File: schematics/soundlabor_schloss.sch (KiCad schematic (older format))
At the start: 18 parts, among them P1 CONN_01X03, P2 CONN_01X02, P3 CONN_01X02, Q1 Q_NMOS_GDS, U1 4538

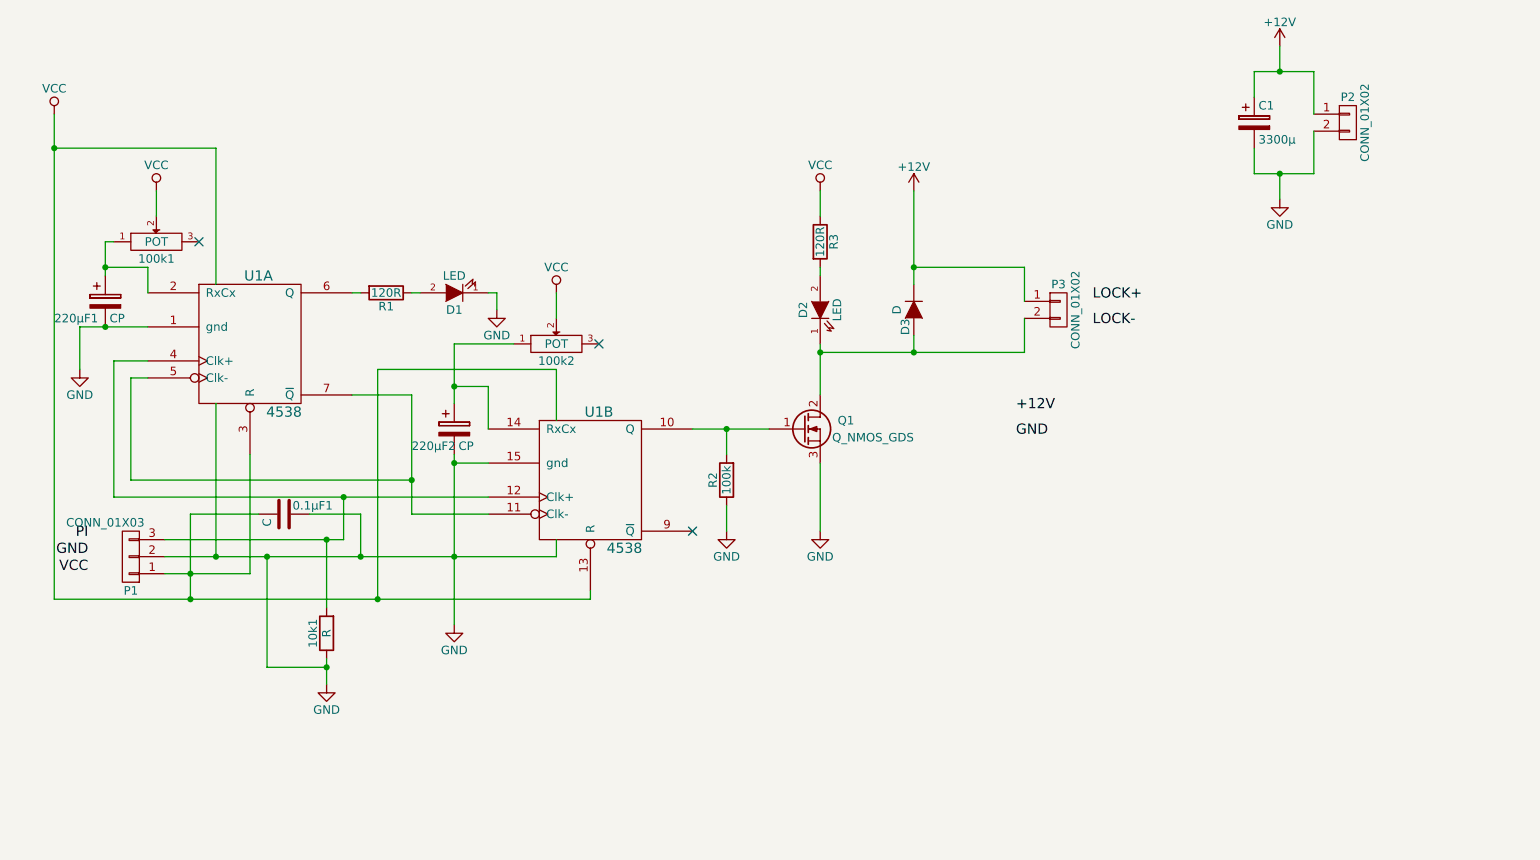
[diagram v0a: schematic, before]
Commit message: final version
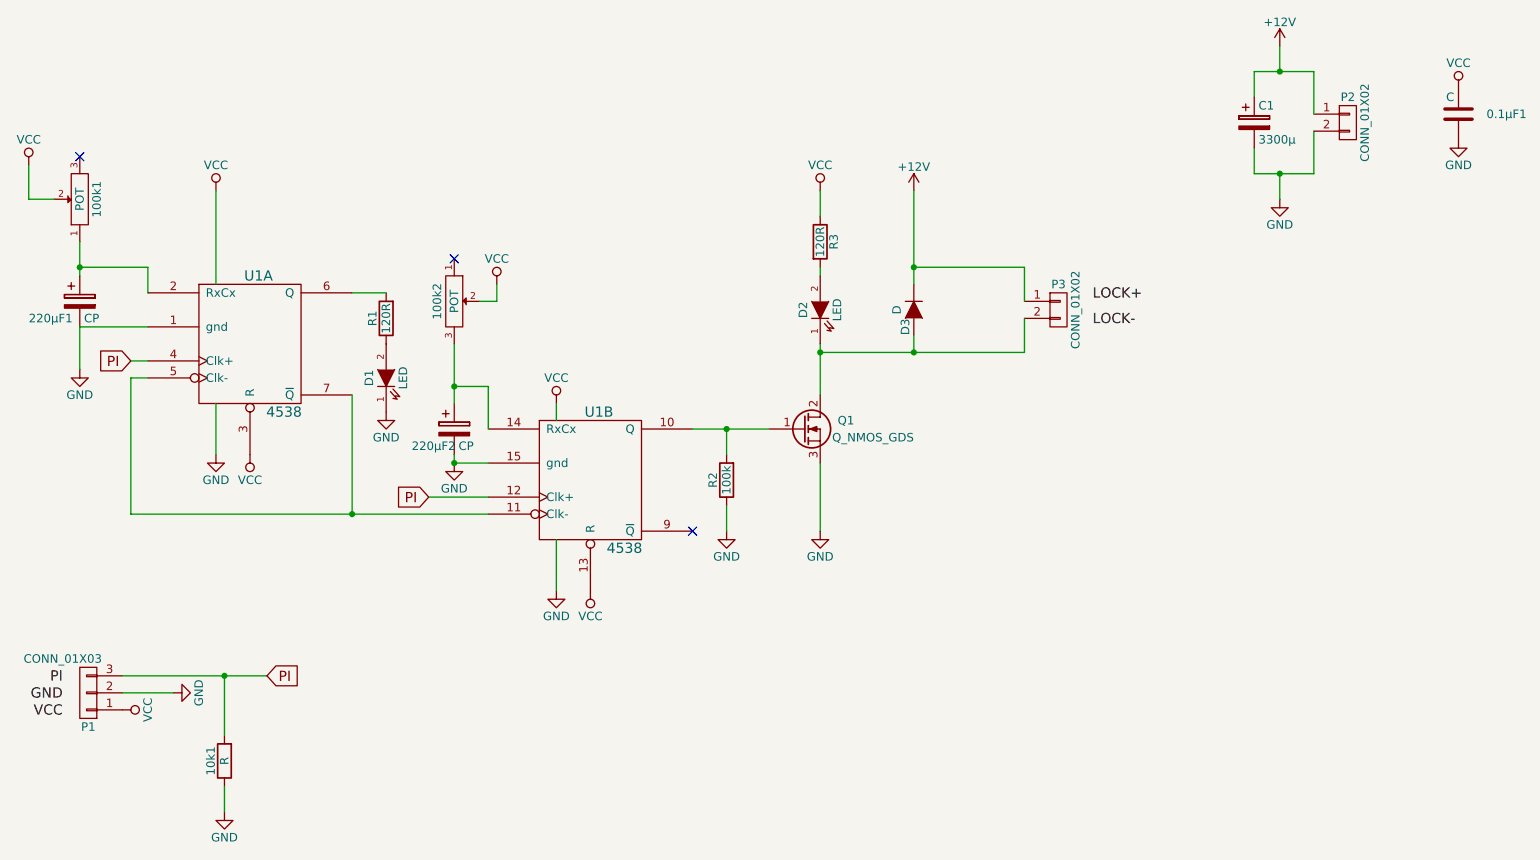
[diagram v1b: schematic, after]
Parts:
- C1: footprint (none) -> raspberrylock_lib:ECA1EM332
- R1, R3: footprint (none) -> Resistors_ThroughHole:Resistor_Horizontal_RM7mm
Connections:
- net PI: now also 10k1.2, P1.3 (P3), U1.12 (Clk+), U1.4 (Clk+)
- net at 220µF2.1, U1.14 (RxCx): now also 100k2.3; no longer 100k2.1
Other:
- moved on the sheet: 0.1µF1, 100k1, 100k2, 10k1, 220µF1, D1, P1, R1
